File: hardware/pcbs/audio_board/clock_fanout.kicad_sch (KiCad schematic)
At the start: 10 parts, among them U6 TAA3040

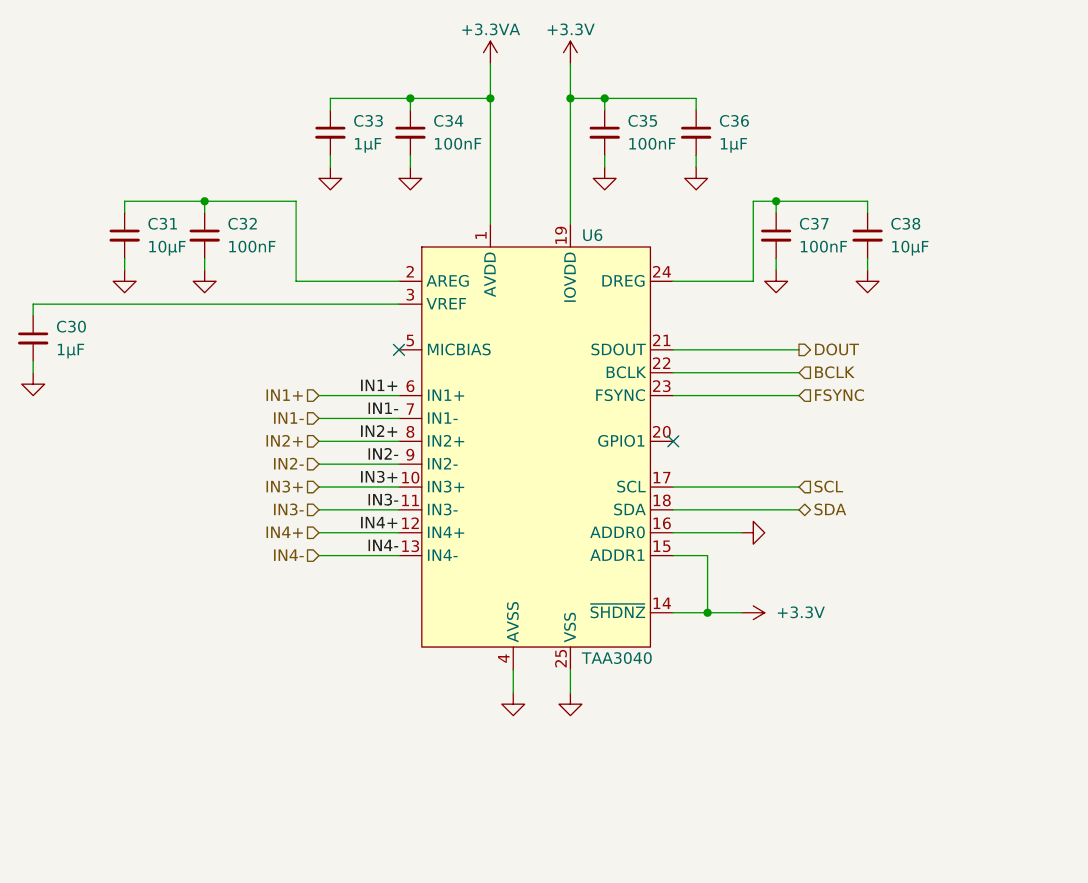
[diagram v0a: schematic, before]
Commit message: prepare for clock fanout
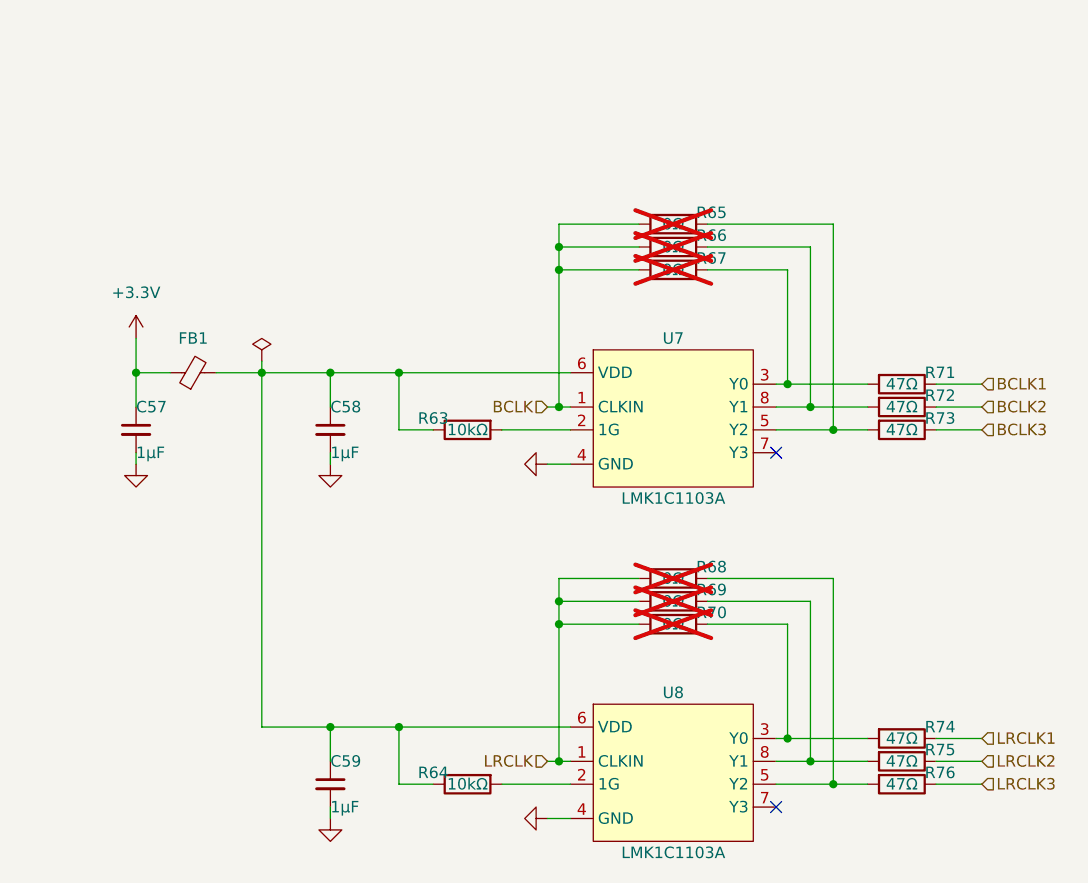
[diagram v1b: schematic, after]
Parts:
- removed C30, C33, C36: 1μF, Capacitor_SMD:C_0805_2012Metric, symbol Device:C_Small
- removed C31, C38: 10μF, Capacitor_SMD:C_0805_2012Metric, symbol Device:C_Small
- removed C32, C34, C35, C37: 100nF, Capacitor_SMD:C_0805_2012Metric, symbol Device:C_Small
- removed U6: TAA3040, ics:WQFN-24-1EP_4x4mm_P0.5mm_EP2.6x2.6mm, symbol audio_ics:TAA3040
- added C57, C58, C59: 1μF, Capacitor_SMD:C_0805_2012Metric, symbol Device:C_Small
- added FB1: FerriteBead_Small, Inductor_SMD:L_0805_2012Metric, symbol Device:FerriteBead_Small
- added R63, R64: 10kΩ, Resistor_SMD:R_0805_2012Metric, symbol Device:R
- added R65, R66, R67, R68, R69, R70: 0Ω, Resistor_SMD:R_0805_2012Metric, symbol Device:R
- added R71, R72, R73, R74, R75, R76: 47Ω, Resistor_SMD:R_0805_2012Metric, symbol Device:R
- added U7, U8: LMK1C1103A, Package_SO:TSSOP-8_4.4x3mm_P0.65mm, symbol ics:LMK1C1104A
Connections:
- net +3.3V: now also C57.1, FB1.1
- net BCLK: now also R65.2, R66.2, R67.2, U7.1 (CLKIN)
- net GND: now also C57.2, C58.2, C59.2, U7.4 (GND), U8.4 (GND)
- new net: C58.1, C59.1, FB1.2, R63.1, R64.1, U7.6 (VDD), U8.6 (VDD)
- new net: R63.2, U7.2 (1G)
- new net: R64.2, U8.2 (1G)
- new net: R70.1, R74.2, U8.3 (Y0)
- new net: R68.1, R76.2, U8.5 (Y2)
- new net: R69.1, R75.2, U8.8 (Y1)
- new net: R66.1, R72.2, U7.8 (Y1)
- new net: R65.1, R73.2, U7.5 (Y2)
- new net: R67.1, R71.2, U7.3 (Y0)
- new net BCLK1: R71.1
- new net BCLK2: R72.1
- new net BCLK3: R73.1
- new net LRCLK: R68.2, R69.2, R70.2, U8.1 (CLKIN)
- new net LRCLK1: R74.1
- new net LRCLK2: R75.1
- new net LRCLK3: R76.1
